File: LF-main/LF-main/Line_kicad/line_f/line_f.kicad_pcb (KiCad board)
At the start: 2 copper layers, 135 x 150 mm, 15 parts, among them M2 Motor_DC, M3 Motor_DC, SW1 SW_SPST, SW2 SW_SPDT, SW3 SW_Push, SW4 SW_Push, U1 TB6612FNG_LINE, m1 BLACKPILL

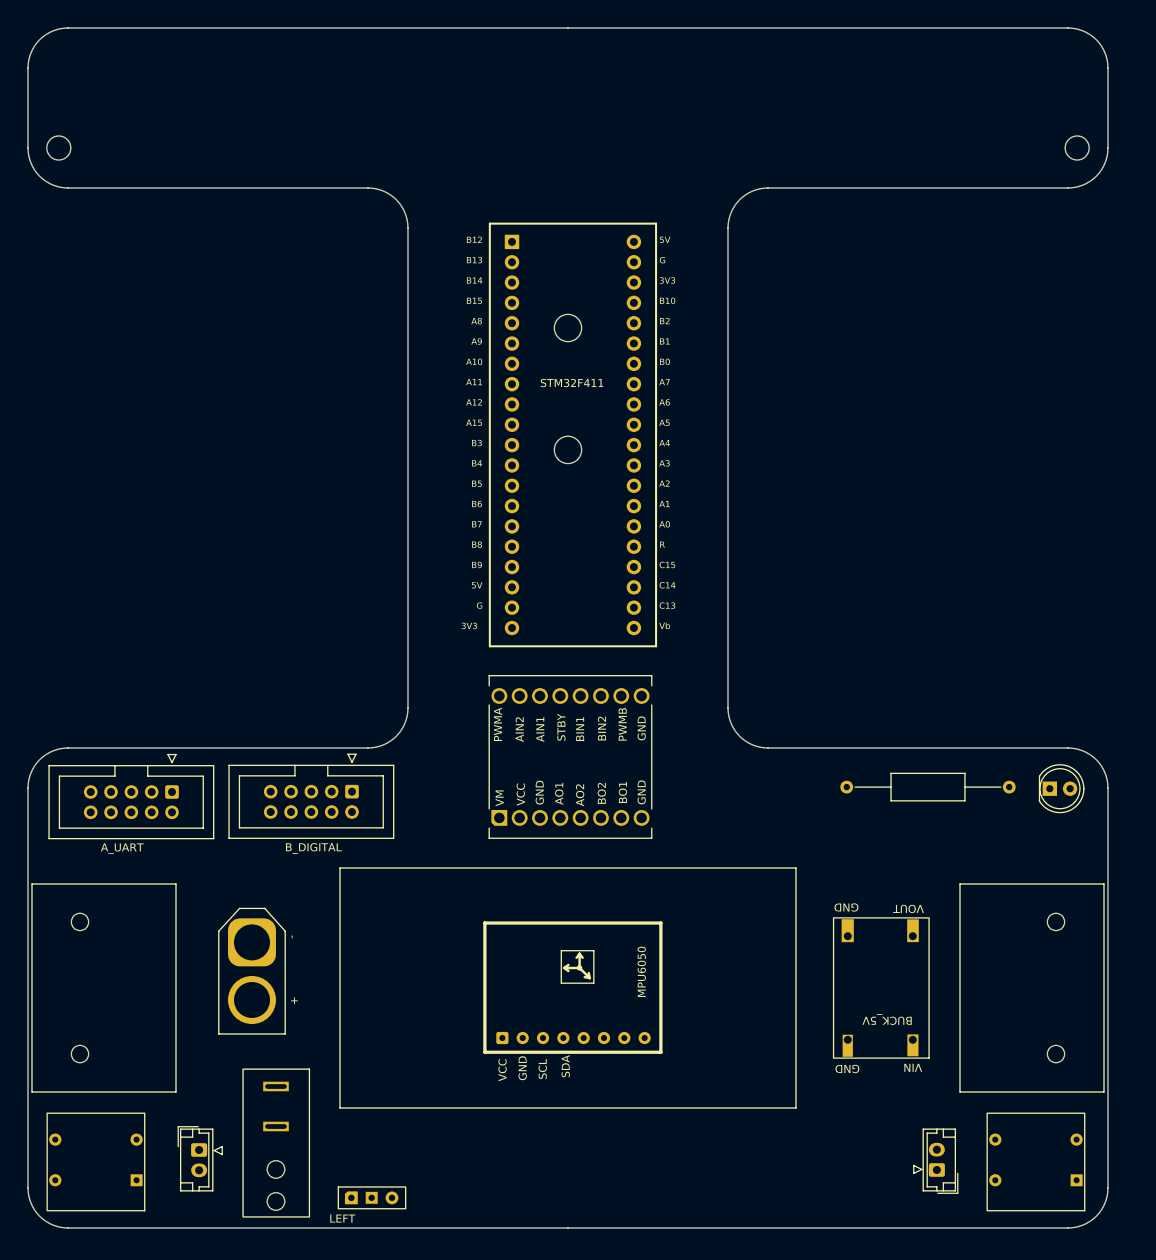
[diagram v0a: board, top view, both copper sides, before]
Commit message: 7battery-center#
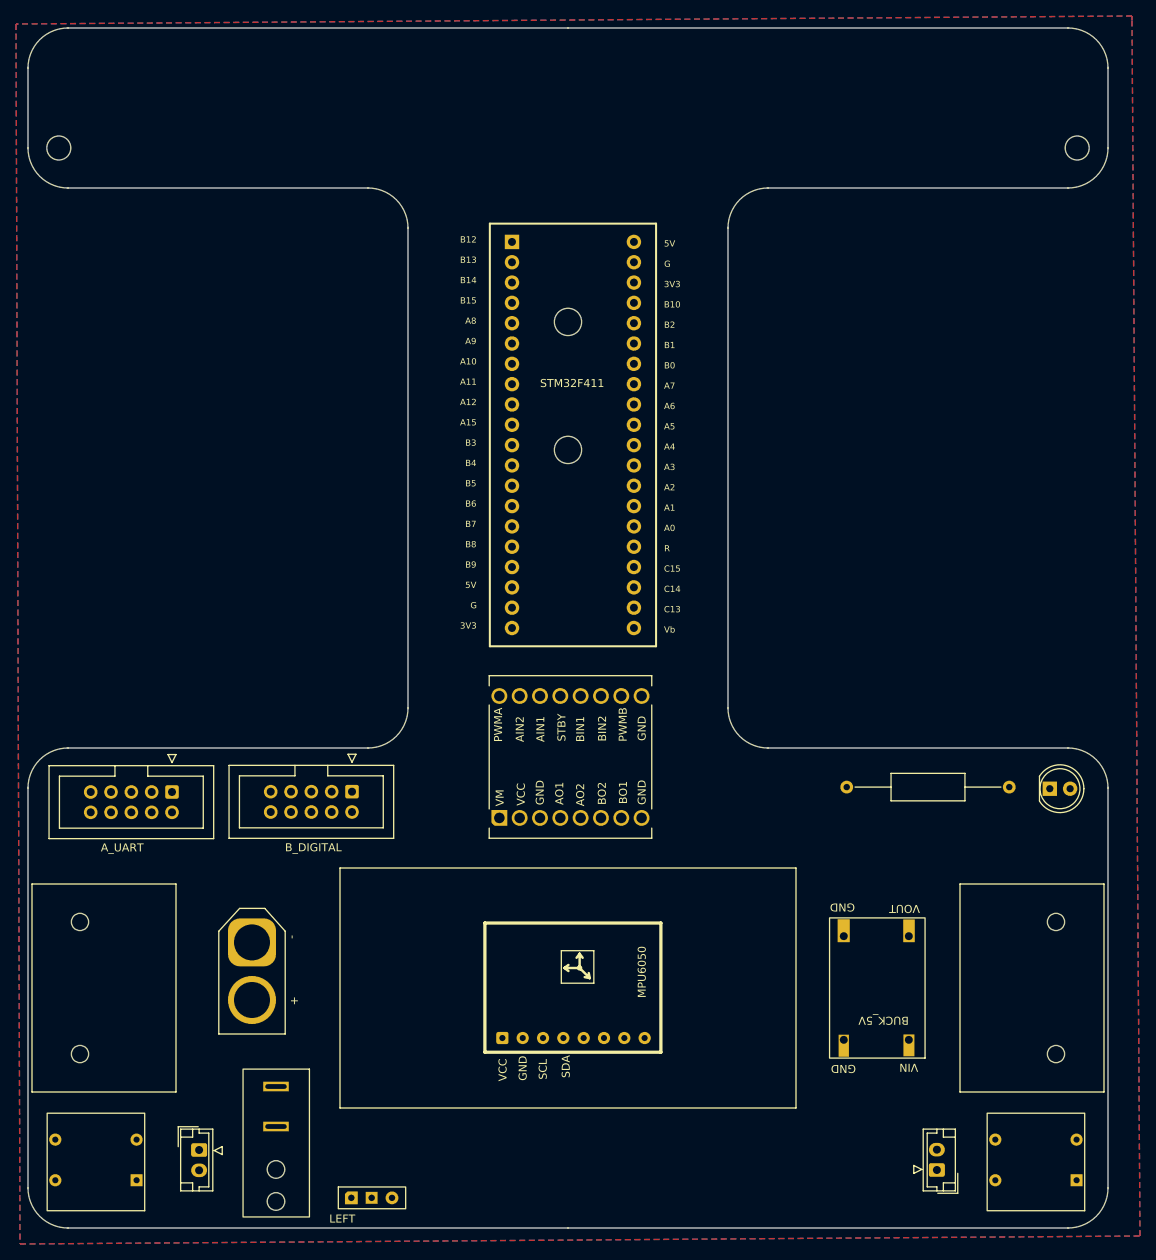
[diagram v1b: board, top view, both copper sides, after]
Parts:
- moved BUCK1 0.50 mm to (112.8, 138.4)
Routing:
- added copper zone on B.Cu, net C_GND
- added copper zone on F.Cu, net C_GND
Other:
- outline, holes or cut-outs redrawn
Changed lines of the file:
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@@
 	(footprint "LINE_F_FOOT_LIB:BUCK_SMD"
 		(layer "F.Cu")
-		(at 113.3375 138.437 180)
+		(at 112.8375 138.437 180)
 		(property "Reference" "BUCK1"
 			(at -11.1625 -3.563 180)
@@
 		)
 		(fp_text user "A11"
-			(at -13.3609 -7.03384 0)
+			(at -14.12 -7.09 0)
 			(unlocked yes)
 			(layer "F.SilkS")
@@
 		)
 		(fp_text user "A9"
-			(at -12.7142 -12.11384 0)
+			(at -13.4733 -12.17 0)
 			(unlocked yes)
 			(layer "F.SilkS")
@@
 		)
 		(fp_text user "A15"
-			(at -13.3609 -1.95384 0)
+			(at -14.12 -2.01 0)
 			(unlocked yes)
 			(layer "F.SilkS")
@@
 		)
 		(fp_text user "3V3"
-			(at -13.9959 23.44616 0)
+			(at -14.12 23.39 0)
 			(unlocked yes)
 			(layer "F.SilkS")
@@
 		)
 		(fp_text user "A1"
-			(at 10.7808 8.20616 0)
+			(at 11.38 8.65 0)
 			(unlocked yes)
 			(layer "F.SilkS")
@@
 		)
 		(fp_text user "B14"
-			(at -13.3609 -19.73384 0)
+			(at -14.12 -19.79 0)
 			(unlocked yes)
 			(layer "F.SilkS")
@@
 		)
 		(fp_text user "C13"
-			(at 10.7691 20.90616 0)
+			(at 11.3683 21.35 0)
 			(unlocked yes)
 			(layer "F.SilkS")
@@
 		)
 		(fp_text user "A5"
-			(at 10.7808 -1.95384 0)
+			(at 11.38 -1.51 0)
 			(unlocked yes)
 			(layer "F.SilkS")
@@
 		)
 		(fp_text user "B4"
-			(at -12.7142 3.12616 0)
+			(at -13.4733 3.07 0)
 			(unlocked yes)
 			(layer "F.SilkS")
@@
 		)
 		(fp_text user "R"
-			(at 10.795 13.29248 0)
+			(at 11.3942 13.73632 0)
 			(unlocked yes)
 			(layer "F.SilkS")
@@
 		)
 		(fp_text user "A3"
-			(at 10.7808 3.12616 0)
+			(at 11.38 3.57 0)
 			(unlocked yes)
 			(layer "F.SilkS")
@@
 		)
 		(fp_text user "B9"
-			(at -12.7142 15.82616 0)
+			(at -13.4733 15.77 0)
 			(unlocked yes)
 			(layer "F.SilkS")
@@
 		)
 		(fp_text user "B5"
-			(at -12.7142 5.66616 0)
+			(at -13.4733 5.61 0)
 			(unlocked yes)
 			(layer "F.SilkS")
@@
 		)
 		(fp_text user "B13"
-			(at -13.3609 -22.27384 0)
+			(at -14.12 -22.33 0)
 			(unlocked yes)
 			(layer "F.SilkS")
@@
 		)
 		(fp_text user "Vb"
-			(at 10.7808 23.44616 0)
+			(at 11.38 23.89 0)
 			(unlocked yes)
 			(layer "F.SilkS")
@@
 		)
 		(fp_text user "B3"
-			(at -12.7142 0.58616 0)
+			(at -13.4733 0.53 0)
 			(unlocked yes)
 			(layer "F.SilkS")
@@
 		)
 		(fp_text user "C15"
-			(at 10.7691 15.82616 0)
+			(at 11.3683 16.27 0)
 			(unlocked yes)
 			(layer "F.SilkS")
@@
 		)
 		(fp_text user "A4"
-			(at 10.7808 0.58616 0)
+			(at 11.38 1.03 0)
 			(unlocked yes)
 			(layer "F.SilkS")
@@
 		)
 		(fp_text user "5V"
-			(at 10.7808 -24.81384 0)
+			(at 11.38 -24.37 0)
 			(unlocked yes)
 			(layer "F.SilkS")
@@
 		)
 		(fp_text user "B8"
-			(at -12.7142 13.28616 0)
+			(at -13.4733 13.23 0)
 			(unlocked yes)
 			(layer "F.SilkS")
@@
 		)
 		(fp_text user "A7"
-			(at 10.7808 -7.03384 0)
+			(at 11.38 -6.59 0)
 			(unlocked yes)
 			(layer "F.SilkS")
@@
 		)
 		(fp_text user "A6"
-			(at 10.7808 -4.49384 0)
+			(at 11.38 -4.05 0)
 			(unlocked yes)
 			(layer "F.SilkS")
@@
 		)
 		(fp_text user "B6"
-			(at -12.7142 8.20616 0)
+			(at -13.4733 8.15 0)
 			(unlocked yes)
 			(layer "F.SilkS")
@@
 		)
 		(fp_text user "A12"
-			(at -13.3609 -4.49384 0)
+			(at -14.12 -4.55 0)
 			(unlocked yes)
 			(layer "F.SilkS")
@@
 		)
 		(fp_text user "G"
-			(at -12.065 20.91248 0)
+			(at -12.8241 20.85632 0)
 			(unlocked yes)
 			(layer "F.SilkS")
@@
 		)
 		(fp_text user "B12"
-			(at -13.3609 -24.81384 0)
+			(at -14.12 -24.87 0)
 			(unlocked yes)
 			(layer "F.SilkS")
@@
 		)
 		(fp_text user "A10"
-			(at -13.3609 -9.57384 0)
+			(at -14.12 -9.63 0)
 			(unlocked yes)
 			(layer "F.SilkS")
@@
 		)
 		(fp_text user "A0"
-			(at 10.7808 10.74616 0)
+			(at 11.38 11.19 0)
 			(unlocked yes)
 			(layer "F.SilkS")
@@
 		)
 		(fp_text user "B10"
-			(at 10.7691 -17.19384 0)
+			(at 11.3683 -16.75 0)
 			(unlocked yes)
 			(layer "F.SilkS")
@@
 		)
 		(fp_text user "G"
-			(at 10.795 -22.26752 0)
+			(at 11.3942 -21.82368 0)
 			(unlocked yes)
 			(layer "F.SilkS")
@@
 		)
 		(fp_text user "A8"
-			(at -12.7142 -14.65384 0)
+			(at -13.4733 -14.71 0)
 			(unlocked yes)
 			(layer "F.SilkS")
@@
 		)
 		(fp_text user "B2"
-			(at 10.7808 -14.65384 0)
+			(at 11.38 -14.21 0)
 			(unlocked yes)
 			(layer "F.SilkS")
@@
 		)
 		(fp_text user "C14"
-			(at 10.7691 18.36616 0)
+			(at 11.3683 18.81 0)
 			(unlocked yes)
 			(layer "F.SilkS")
@@
 		)
 		(fp_text user "B1"
-			(at 10.7808 -12.11384 0)
+			(at 11.38 -11.67 0)
 			(unlocked yes)
 			(layer "F.SilkS")
@@
 		)
 		(fp_text user "B7"
-			(at -12.7142 10.74616 0)
+			(at -13.4733 10.69 0)
 			(unlocked yes)
 			(layer "F.SilkS")
@@
 		)
 		(fp_text user "B15"
-			(at -13.3609 -17.19384 0)
+			(at -14.12 -17.25 0)
 			(unlocked yes)
 			(layer "F.SilkS")
@@
 		)
 		(fp_text user "5V"
-			(at -12.7142 18.36616 0)
+			(at -13.4733 18.31 0)
 			(unlocked yes)
 			(layer "F.SilkS")
@@
 		)
 		(fp_text user "B0"
-			(at 10.7808 -9.57384 0)
+			(at 11.38 -9.13 0)
 			(unlocked yes)
 			(layer "F.SilkS")
@@
 		)
 		(fp_text user "A2"
-			(at 10.7808 5.66616 0)
+			(at 11.38 6.11 0)
 			(unlocked yes)
 			(layer "F.SilkS")
@@
 		)
 		(fp_text user "3V3"
-			(at 10.7691 -19.73384 0)
+			(at 11.3683 -19.29 0)
 			(unlocked yes)
 			(layer "F.SilkS")
@@
 	)
 	(gr_circle
-		(center 87.5 59.5)
-		(end 89.024 58.738)
+		(center 87.5 58.74)
+		(end 89.203884 58.74)
 		(stroke
 			(width 0.05)
-			(type default)
+			(type solid)
 		)
 		(fill no)
@@
 		(layer "Edge.Cuts")
 	)
+	(zone
+		(net 1)
+		(net_name "C_GND")
+		(layers "F.Cu" "B.Cu")
+		(hatch edge 0.5)
+		(connect_pads
+			(clearance 0.5)
+		)
+		(min_thickness 0.25)
+		(filled_areas_thickness no)
+		(fill yes
+			(thermal_gap 0.5)
+			(thermal_bridge_width 0.5)
+		)
+		(polygon
+			(pts
+				(xy 18.5 21.5) (xy 19 174) (xy 159 173) (xy 158 21) (xy 158 20.5)
+			)
+		)
+	)
 	(group ""
